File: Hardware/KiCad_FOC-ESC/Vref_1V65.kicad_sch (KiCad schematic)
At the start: 1 part

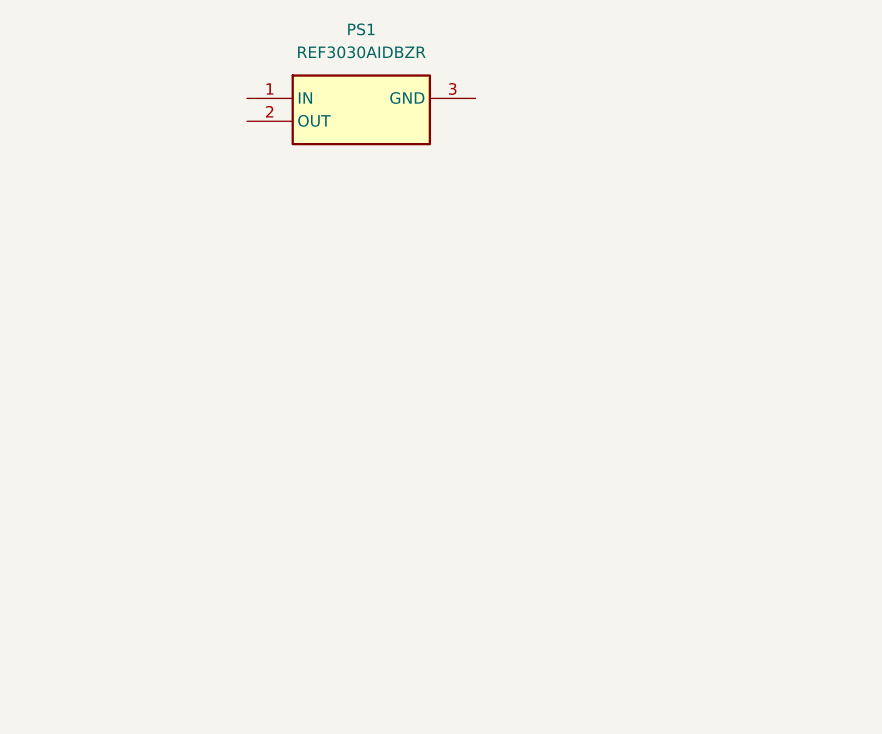
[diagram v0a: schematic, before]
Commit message: initial connections
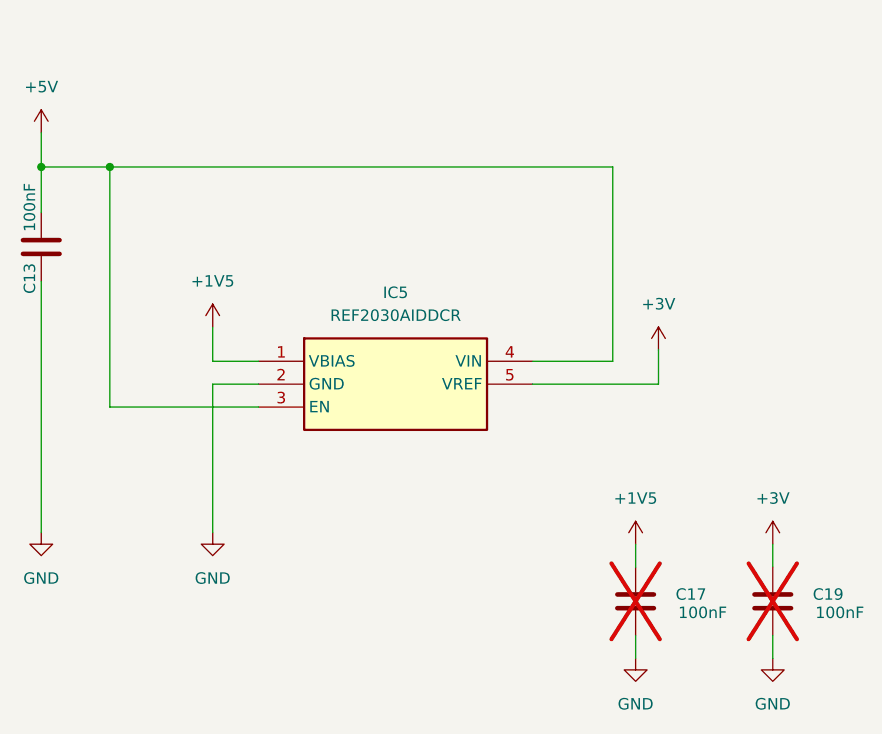
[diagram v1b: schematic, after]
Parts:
- removed PS1: REF3030AIDBZR, SamacSys_Parts:SOT96P240X105-3N, symbol SamacSys_Parts:REF3030AIDBZR
- added C13, C17, C19: 100nF, Capacitor_SMD:C_0402_1005Metric, symbol Device:C
- added IC5: REF2030AIDDCR, SOT95P280X110-5N, symbol SamacSys_Parts:REF2030AIDDCR
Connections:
- new net +1V5: C17.2, IC5.1 (VBIAS)
- new net +3V: C19.2, IC5.5 (VREF)
- new net +5V: C13.2, IC5.3 (EN), IC5.4 (VIN)
- new net GND: C13.1, C17.1, C19.1, IC5.2 (GND)
